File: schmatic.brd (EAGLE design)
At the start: 109.2 x 16.2 mm, 18 parts, among them SW1 SWITCH-SMD-EVQP-P2602W

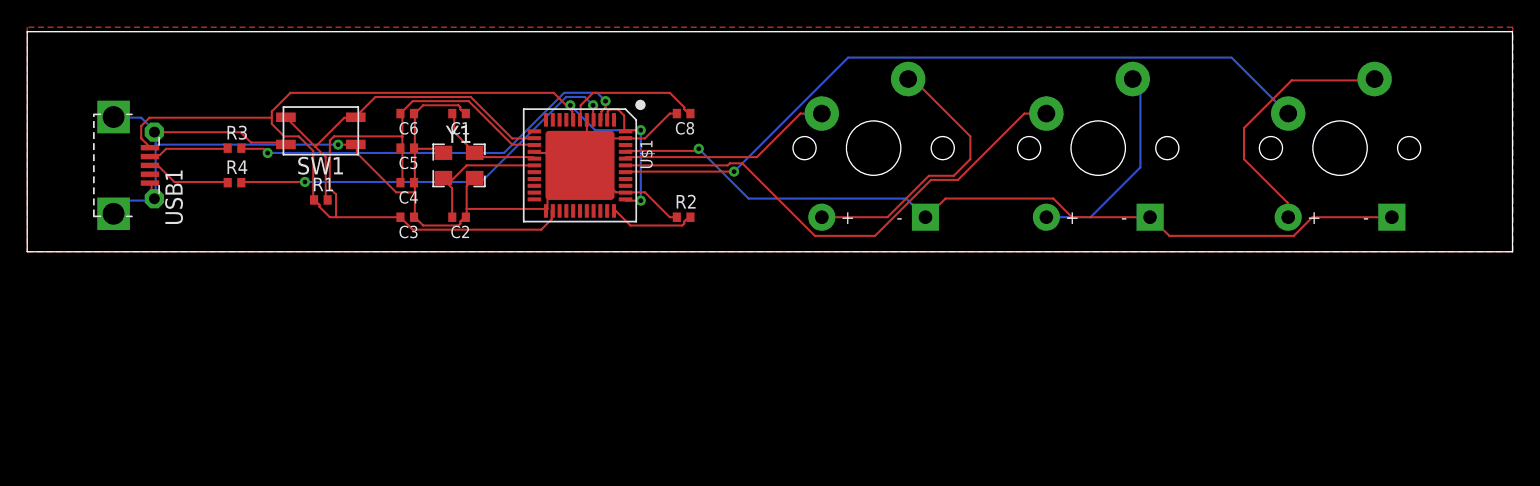
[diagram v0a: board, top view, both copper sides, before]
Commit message: updated based off feedback, included extra osh screenshot
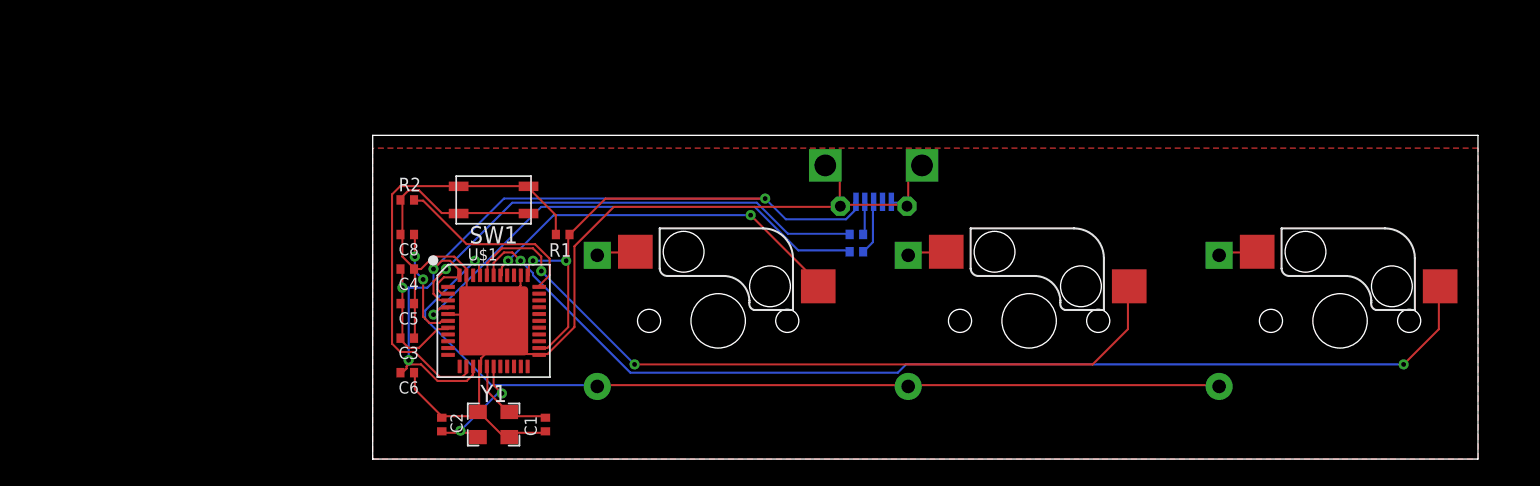
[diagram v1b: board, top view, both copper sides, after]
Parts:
- removed U$2, U$3, U$4: KEYSWITCH-DIODE-MX-1U-DIODE, Keyboard:MX-1U-DIODE
- added D1, D2, D3: 1N4148, Components:DO-35
- added U$5, U$6, U$7: KEYSWITCH-PLAIN-MXHSPCB-1U, Keyboard:MXHSPCB-1U
- moved USB1 53.4 mm to (96.5, 54.6), flipped to the bottom, turned to 270 degrees
- moved R3 46.2 mm to (95.2, 52.1), flipped to the bottom
- moved R4 46.0 mm to (95.2, 50.8), flipped to the bottom
- moved C1 23.7 mm to (72.4, 38.1), turned to 270 degrees
- moved C8 22.2 mm to (62.2, 52.1)
- moved R2 20.4 mm to (62.2, 54.6)
- moved Y1 19.2 mm to (68.6, 38.1)
- moved C6 19.1 mm to (62.2, 41.9)
- moved R1 18.0 mm to (73.7, 52.1), turned to 180 degrees
- moved C2 15.3 mm to (64.8, 38.1), turned to 90 degrees
- moved SW1 13.7 mm to (68.6, 54.6)
- moved U$1 13.1 mm to (68.6, 45.7), turned to 0 degrees
- moved C5 11.4 mm to (62.2, 47.0)
- moved C3 8.89 mm to (62.2, 44.5)
- moved C4 6.35 mm to (62.2, 49.5)
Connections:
- removed net N$11: U$3.D+, U$3.MX2
- removed net N$12: U$4.D+, U$4.MX2
- removed net N$16: U$1.38, U$4.MX1
- new net N$17: D1.A, U$5.MX2
- new net N$18: D2.A, U$6.MX2
- new net N$19: D3.A, U$7.MX2
- net N$13: now also D1.C, D2.C, D3.C; no longer U$2.D-, U$3.D-, U$4.D-
- net N$14: now also U$5.MX1; no longer U$2.MX1
- net N$15: now also U$1.38, U$7.MX1; no longer U$1.39, U$3.MX1
- net N$9: now also U$1.39, U$6.MX1; no longer U$2.D+, U$2.MX2
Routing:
- net N$9: track 20.7 -> 79.0 mm, vias 0 -> 2
- net N$16: track 53.9 -> 0.00 mm, vias 1 -> 0
- net N$14: track 15.8 -> 56.9 mm, vias 0 -> 2
- net N$12: track 19.1 -> 0.00 mm
- net N$11: track 15.2 -> 0.00 mm
- net VCC: track 108.8 -> 95.9 mm, vias 3 -> 6
- net N$15: track 36.9 -> 27.9 mm, vias 0 -> 2
- net N$4: track 6.40 -> 14.1 mm
- net N$13: track 60.8 -> 67.8 mm
- net N$7: track 29.8 -> 36.6 mm, vias 2 -> 1
- net N$3: track 26.3 -> 32.7 mm
- net N$6: track 30.6 -> 36.1 mm, vias 2 -> 1
- net N$5: track 5.96 -> 2.48 mm
- net GND: track 103.0 -> 106.4 mm, vias 1 -> 0
- net N$19: track 0.00 -> 2.94 mm
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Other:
- board size 109.2 x 16.2 mm -> 81.3 x 23.8 mm
